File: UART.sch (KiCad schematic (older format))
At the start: 9 parts

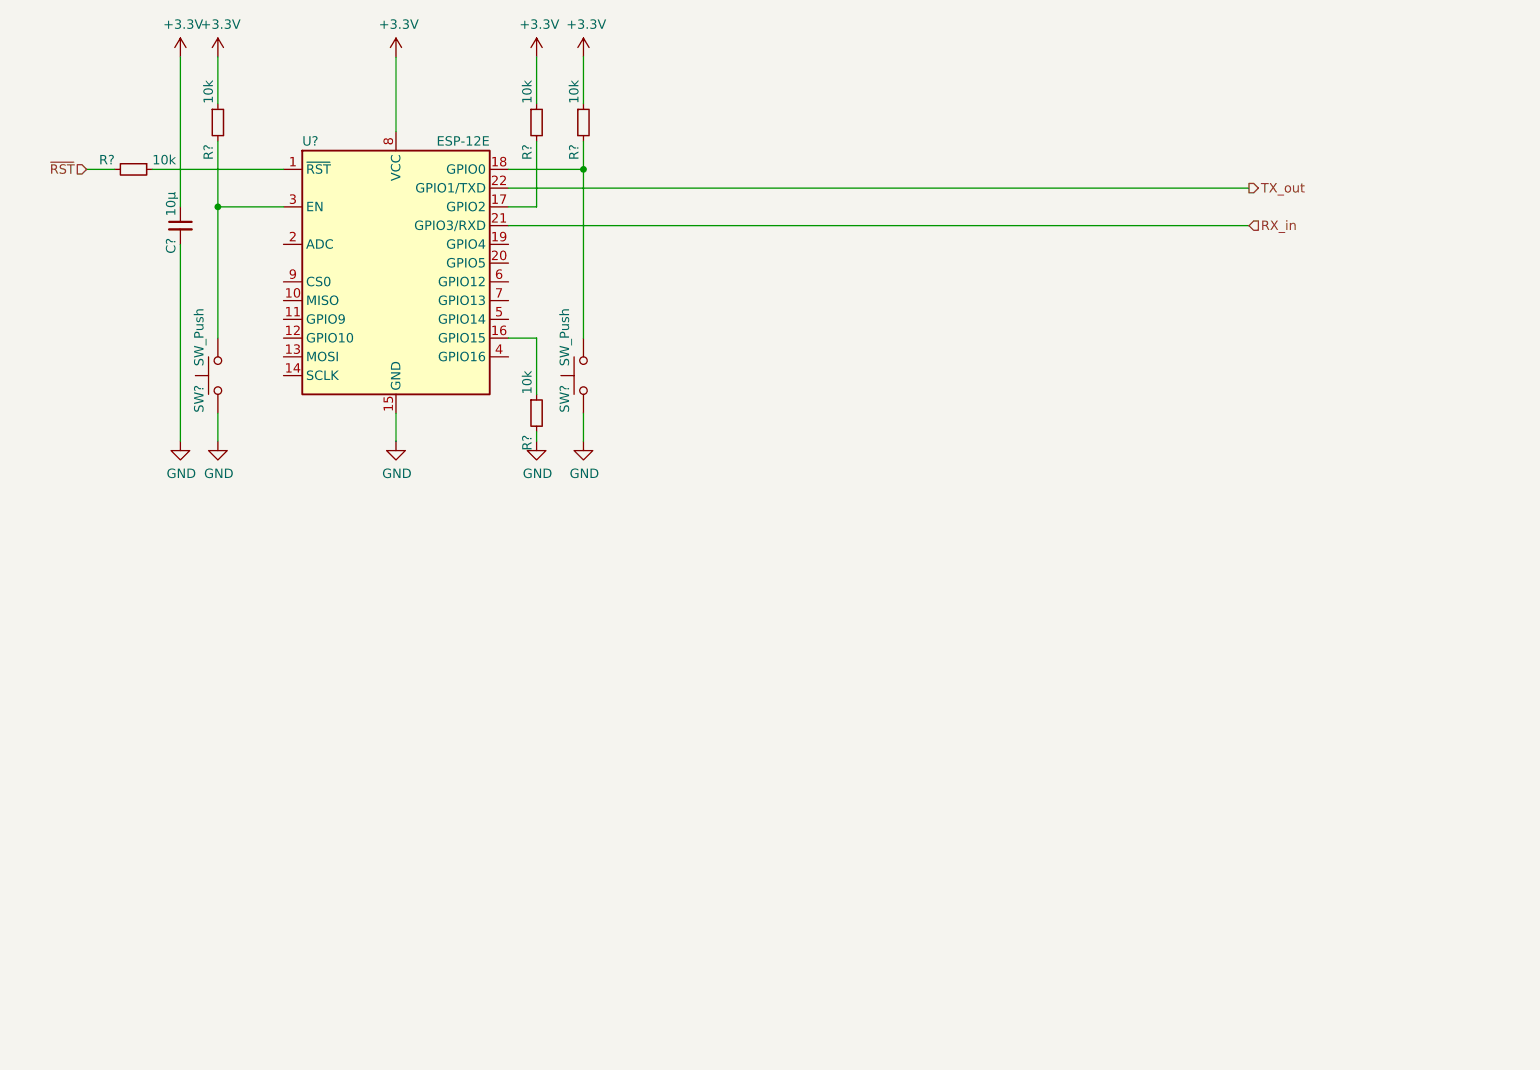
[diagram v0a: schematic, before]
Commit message: Erste fertige Version
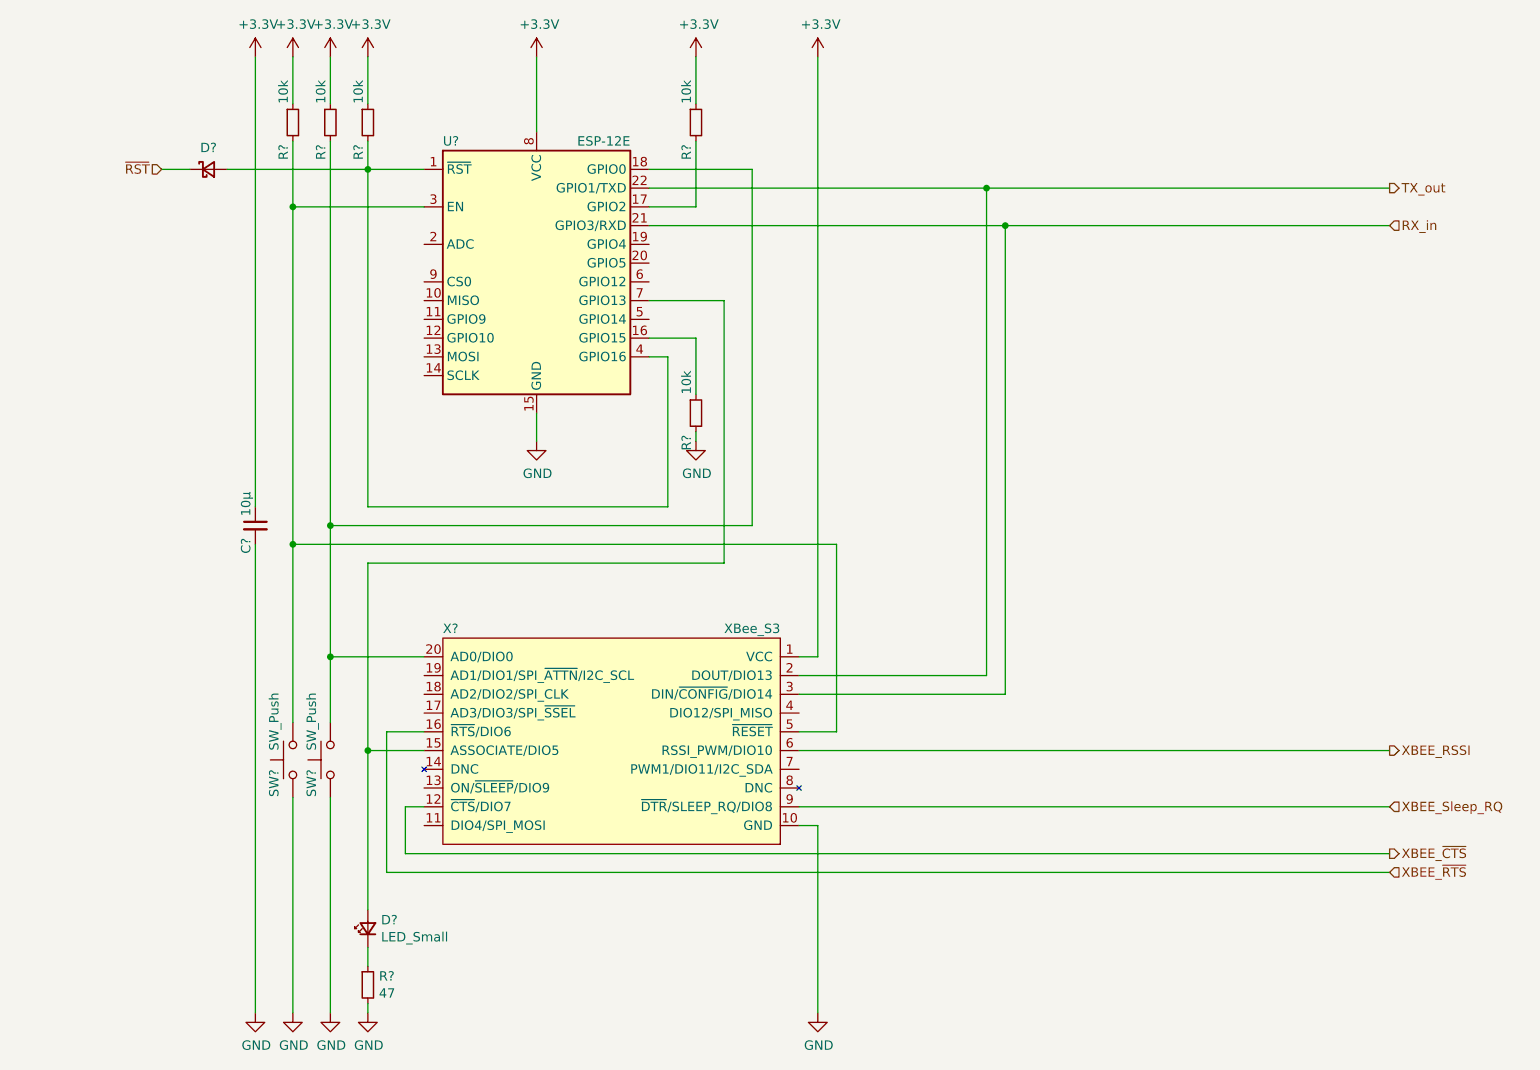
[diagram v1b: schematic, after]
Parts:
- removed R?: 10k, symbol Device:R_Small
- added D?: LED_Small, symbol Device:LED_Small
- added D?: D_Schottky_Small, symbol Device:D_Schottky_Small
- added R?: 47, symbol Device:R_Small
- added R?: 10k, symbol Device:R_Small
- added X?: XBee_S3, symbol HS-Wismar:XBee_S3
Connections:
- net +3V3: now also R?.1, X?.1 (VCC)
- net GND: now also R?.2, X?.10 (GND)
- net RX_in: now also X?.3 (DIN/~CONFIG~/DIO14)
- net TX_out: now also X?.2 (DOUT/DIO13)
- net ~RST: now also D?.1 (K)
- net at U?.1 (~RST): now also U?.4 (GPIO16), D?.2 (A), R?.2
- net at R?.2, SW?.2, U?.18 (GPIO0): now also X?.20 (AD0/DIO0)
- net at R?.2, SW?.2, U?.3 (EN): now also X?.5 (~RESET)
- net at U?.7 (GPIO13): now also D?.2 (A), X?.15 (ASSOCIATE/DIO5)
- new net: D?.1 (K), R?.1
- new net XBEE_RSSI: X?.6 (RSSI_PWM/DIO10)
- new net XBEE_Sleep_RQ: X?.9 (~DTR~/SLEEP_RQ/DIO8)
- new net XBEE_~CTS~: X?.12 (~CTS~/DIO7)
- new net XBEE_~RTS~: X?.16 (~RTS~/DIO6)
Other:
- moved on the sheet: C?, R?, SW?, U?

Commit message: Externe Spannungsversorgung
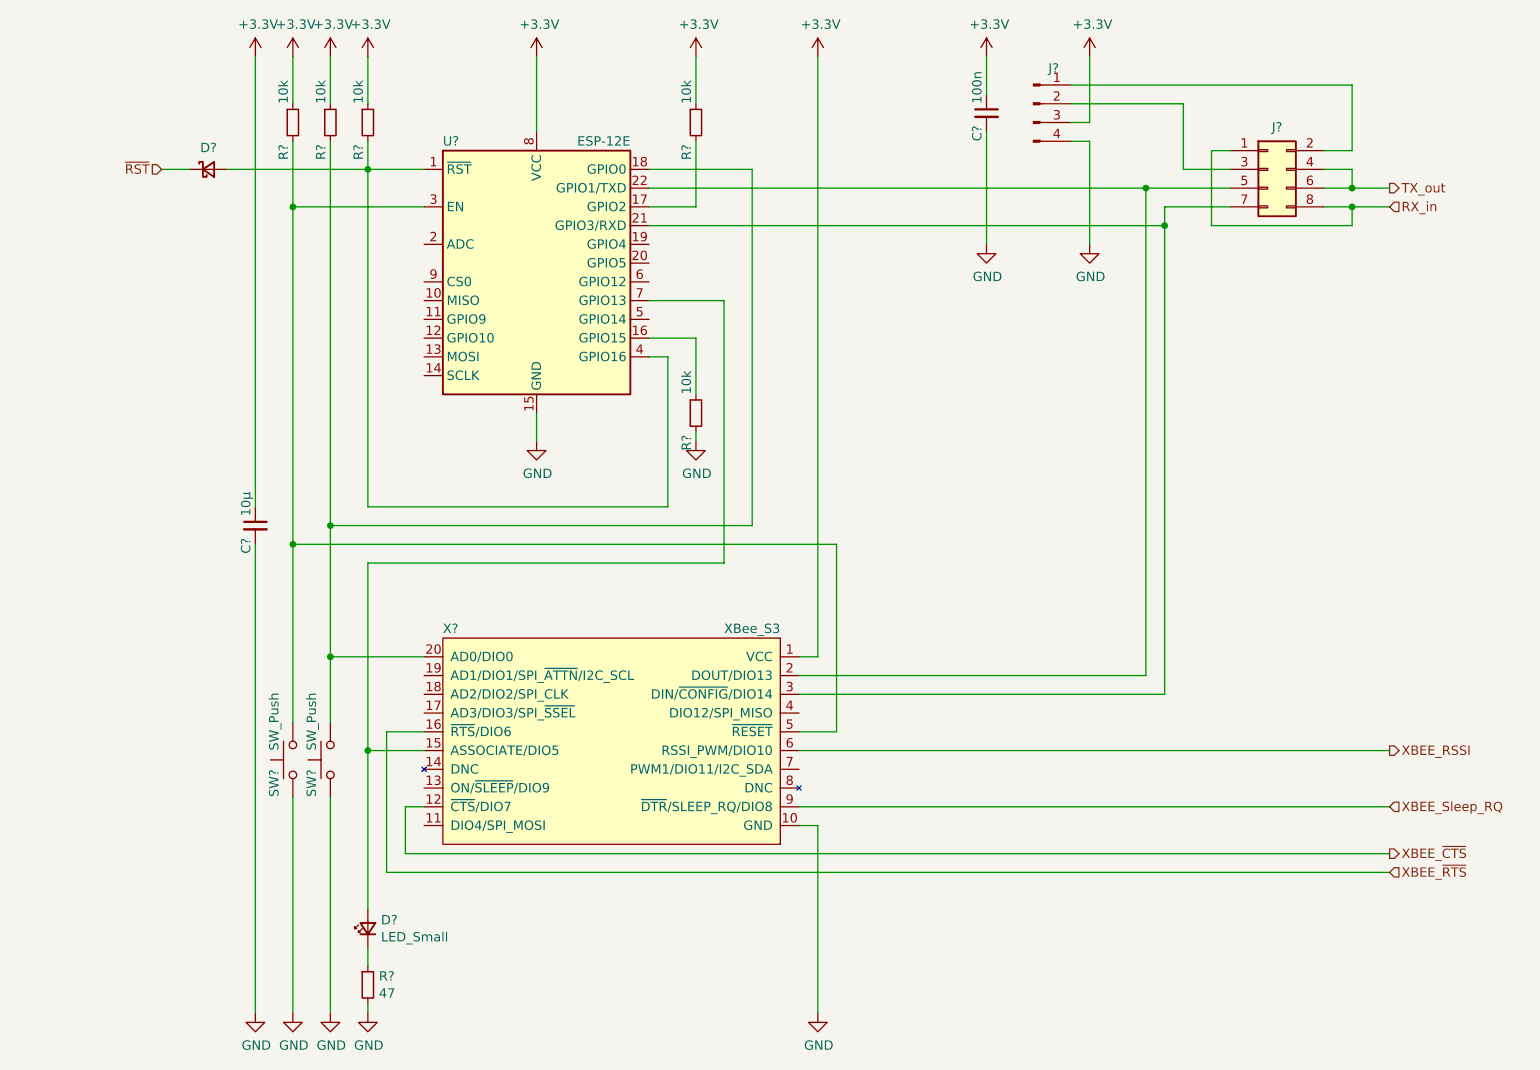
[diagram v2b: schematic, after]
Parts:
- added C?: 100n, symbol Device:C_Small
- added J?: Conn_01x04_Male, symbol Connector:Conn_01x04_Male
- added J?: Conn_02x04_Odd_Even, symbol Connector_Generic:Conn_02x04_Odd_Even
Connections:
- net +3V3: now also C?.1, J?.3 (Pin_3)
- net GND: now also C?.2, J?.4 (Pin_4)
- net RX_in: now also J?.1 (Pin_1), J?.8 (Pin_8); no longer U?.21 (GPIO3/RXD), X?.3 (DIN/~CONFIG~/DIO14)
- net TX_out: now also J?.4 (Pin_4), J?.6 (Pin_6); no longer U?.22 (GPIO1/TXD), X?.2 (DOUT/DIO13)
- new net: J?.7 (Pin_7), U?.21 (GPIO3/RXD), X?.3 (DIN/~CONFIG~/DIO14)
- new net: J?.5 (Pin_5), U?.22 (GPIO1/TXD), X?.2 (DOUT/DIO13)
- new net: J?.1 (Pin_1), J?.2 (Pin_2)
- new net: J?.2 (Pin_2), J?.3 (Pin_3)
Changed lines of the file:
@@
 	0    -1   -1   0
 $EndComp
-Text HLabel 7800 2300 2    50   Input ~ 0
+Text HLabel 7800 2200 2    50   Input ~ 0
 RX_in
 Text HLabel 7800 2100 2    50   Output ~ 0
 TX_out
 Wire Wire Line
-	3850 2100 5650 2100
-Wire Wire Line
-	7800 2300 5750 2300
+	3850 2100 6500 2100
 $Comp
 L power:GND #PWR?
@@
 $EndComp
 Wire Wire Line
-	5650 2100 5650 4700
-Wire Wire Line
-	5650 4700 4650 4700
-Connection ~ 5650 2100
-Wire Wire Line
-	5650 2100 7800 2100
-Wire Wire Line
-	4650 4800 5750 4800
-Wire Wire Line
-	5750 4800 5750 2300
-Connection ~ 5750 2300
-Wire Wire Line
-	5750 2300 3850 2300
+	6500 2100 6500 4700
+Wire Wire Line
+	6500 4700 4650 4700
+Connection ~ 6500 2100
+Wire Wire Line
+	6500 2100 6950 2100
+Wire Wire Line
+	4650 4800 6600 4800
+Wire Wire Line
+	6600 4800 6600 2300
+Wire Wire Line
+	6600 2300 3850 2300
 $Comp
 L power:GND #PWR?
@@
 Wire Wire Line
 	2350 1850 2350 2000
+$Comp
+L Connector:Conn_01x04_Male J?
+U 1 1 5EFDB3FD
+P 5900 1650
+F 0 "J?" H 6008 1839 50  0000 C CNN
+F 1 "Conn_01x04_Male" H 6008 1840 50  0001 C CNN
+F 2 "" H 5900 1650 50  0001 C CNN
+F 3 "~" H 5900 1650 50  0001 C CNN
+	1    5900 1650
+	1    0    0    -1
+$EndComp
+$Comp
+L power:+3.3V #PWR?
+U 1 1 5EFE8401
+P 6200 1400
+F 0 "#PWR?" H 6200 1250 50  0001 C CNN
+F 1 "+3.3V" H 6215 1573 50  0000 C CNN
+F 2 "" H 6200 1400 50  0001 C CNN
+F 3 "" H 6200 1400 50  0001 C CNN
+	1    6200 1400
+	1    0    0    -1
+$EndComp
+Wire Wire Line
+	6200 1400 6200 1750
+Wire Wire Line
+	6200 1750 6100 1750
+$Comp
+L power:GND #PWR?
+U 1 1 5EFEB0C6
+P 6200 2400
+F 0 "#PWR?" H 6200 2150 50  0001 C CNN
+F 1 "GND" H 6205 2227 50  0000 C CNN
+F 2 "" H 6200 2400 50  0001 C CNN
+F 3 "" H 6200 2400 50  0001 C CNN
+	1    6200 2400
+	1    0    0    -1
+$EndComp
+Wire Wire Line
+	6200 2400 6200 1850
+Wire Wire Line
+	6200 1850 6100 1850
+$Comp
+L Device:C_Small C?
+U 1 1 5EFED216
+P 5650 1700
+F 0 "C?" V 5600 1550 50  0000 L CNN
+F 1 "100n" V 5600 1750 50  0000 L CNN
+F 2 "" H 5650 1700 50  0001 C CNN
+F 3 "~" H 5650 1700 50  0001 C CNN
+	1    5650 1700
+	1    0    0    -1
+$EndComp
+$Comp
+L power:+3.3V #PWR?
+U 1 1 5EFEE6C3
+P 5650 1400
+F 0 "#PWR?" H 5650 1250 50  0001 C CNN
+F 1 "+3.3V" H 5665 1573 50  0000 C CNN
+F 2 "" H 5650 1400 50  0001 C CNN
+F 3 "" H 5650 1400 50  0001 C CNN
+	1    5650 1400
+	1    0    0    -1
+$EndComp
+$Comp
+L power:GND #PWR?
+U 1 1 5EFF0343
+P 5650 2400
+F 0 "#PWR?" H 5650 2150 50  0001 C CNN
+F 1 "GND" H 5655 2227 50  0000 C CNN
+F 2 "" H 5650 2400 50  0001 C CNN
+F 3 "" H 5650 2400 50  0001 C CNN
+	1    5650 2400
+	1    0    0    -1
+$EndComp
+Wire Wire Line
+	5650 2400 5650 1800
+Wire Wire Line
+	5650 1600 5650 1400
+$Comp
+L Connector_Generic:Conn_02x04_Odd_Even J?
+U 1 1 5EFF7765
+P 7150 2000
+F 0 "J?" H 7200 2225 50  0000 C CNN
+F 1 "Conn_02x04_Odd_Even" H 7200 2226 50  0001 C CNN
+F 2 "" H 7150 2000 50  0001 C CNN
+F 3 "~" H 7150 2000 50  0001 C CNN
+	1    7150 2000
+	1    0    0    -1
+$EndComp
+Wire Wire Line
+	7450 2100 7600 2100
+Wire Wire Line
+	7800 2200 7600 2200
+Wire Wire Line
+	6950 2200 6600 2200
+Wire Wire Line
+	6600 2200 6600 2300
+Connection ~ 6600 2300
+Wire Wire Line
+	6950 2000 6700 2000
+Wire Wire Line
+	6700 2000 6700 1650
+Wire Wire Line
+	6700 1650 6100 1650
+Wire Wire Line
+	7450 1900 7600 1900
+Wire Wire Line
+	7600 1900 7600 1550
+Wire Wire Line
+	7600 1550 6100 1550
+Wire Wire Line
+	7450 2000 7600 2000
+Wire Wire Line
+	7600 2000 7600 2100
+Connection ~ 7600 2100
+Wire Wire Line
+	7600 2100 7800 2100
+Wire Wire Line
+	7600 2200 7600 2300
+Wire Wire Line
+	7600 2300 6850 2300
+Wire Wire Line
+	6850 2300 6850 1900
+Wire Wire Line
+	6850 1900 6950 1900
+Connection ~ 7600 2200
+Wire Wire Line
+	7600 2200 7450 2200
 $EndSCHEMATC
